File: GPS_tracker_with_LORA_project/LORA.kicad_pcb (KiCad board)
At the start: 2 copper layers, 69.1 x 53.8 mm, 25 parts, among them J1 LoRa Left, J2 Lora Right, J3 ACP test, J4 I2C, J5 Power, U1 LCD, U3 NEO-6M-GPS, U4 24aa32a, U5 A307_3.3V

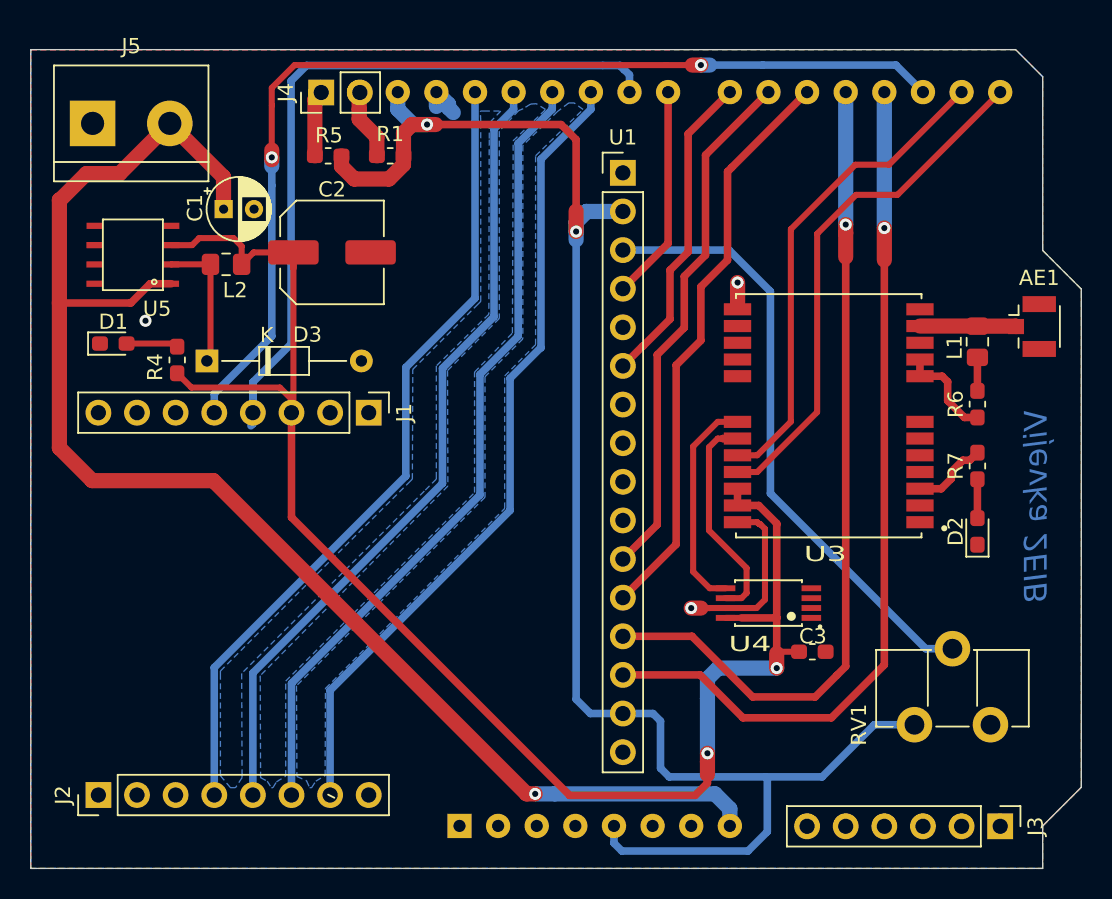
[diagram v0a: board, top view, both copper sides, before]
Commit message: Kursa darbs V2.0
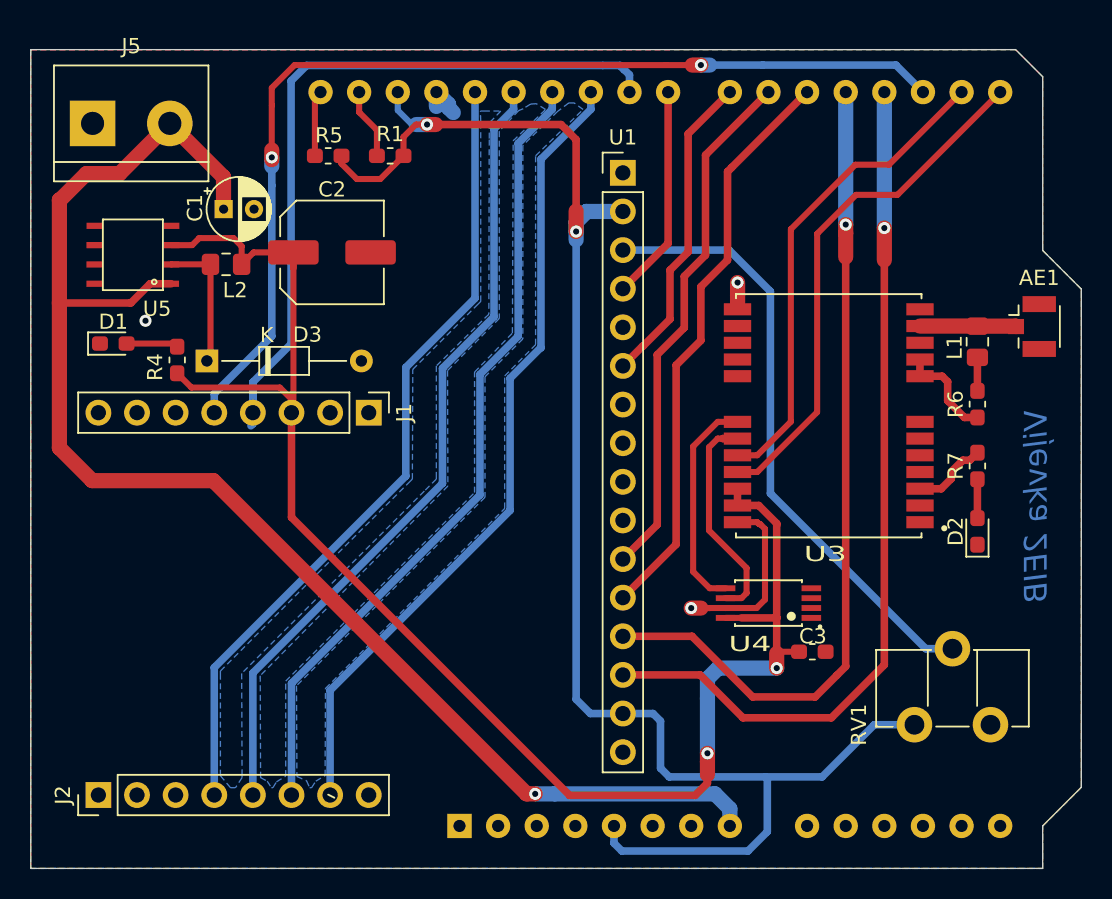
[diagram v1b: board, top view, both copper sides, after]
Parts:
- removed J3: ACP test, Connector_PinHeader_2.54mm:PinHeader_1x06_P2.54mm_Vertical
- removed J4: I2C, Connector_PinHeader_2.54mm:PinHeader_1x02_P2.54mm_Vertical
